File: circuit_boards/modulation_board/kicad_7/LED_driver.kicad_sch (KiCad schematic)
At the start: 11 parts

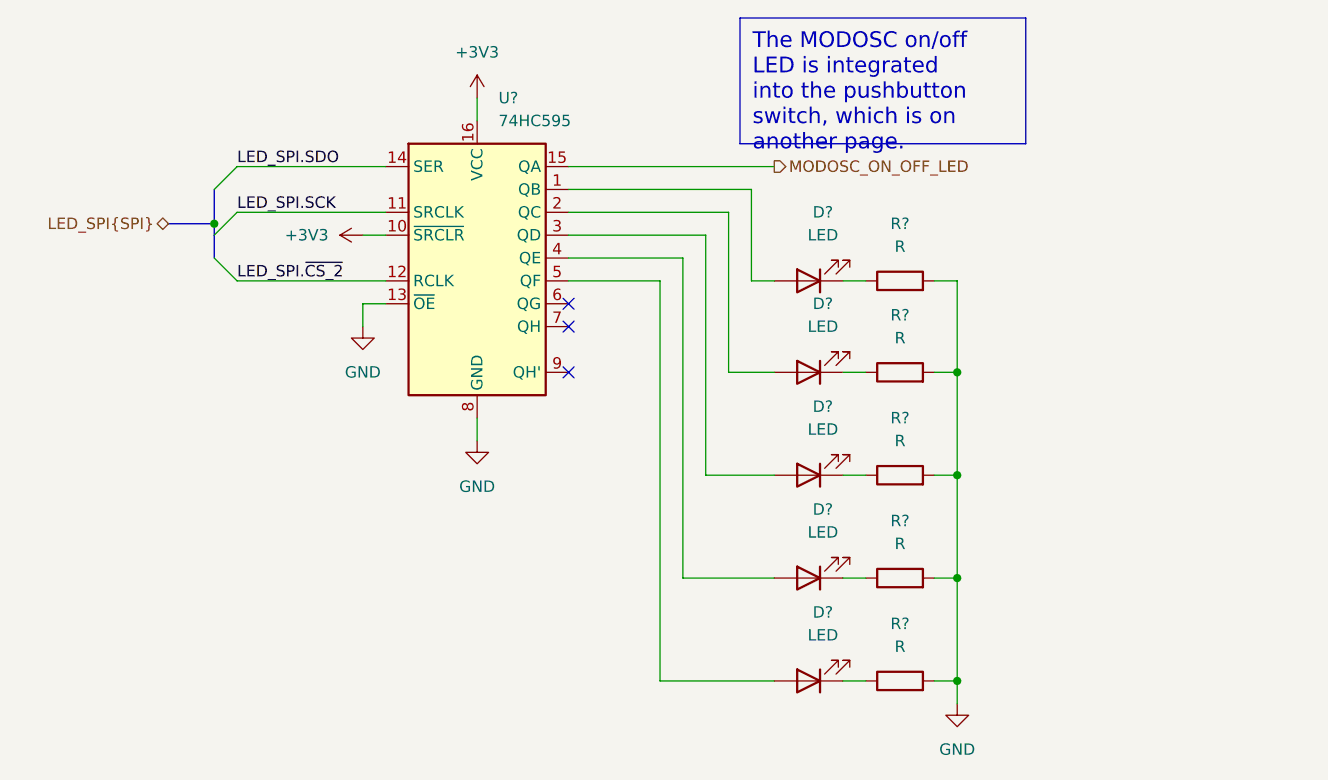
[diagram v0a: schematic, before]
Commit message: Progress on circuit boards
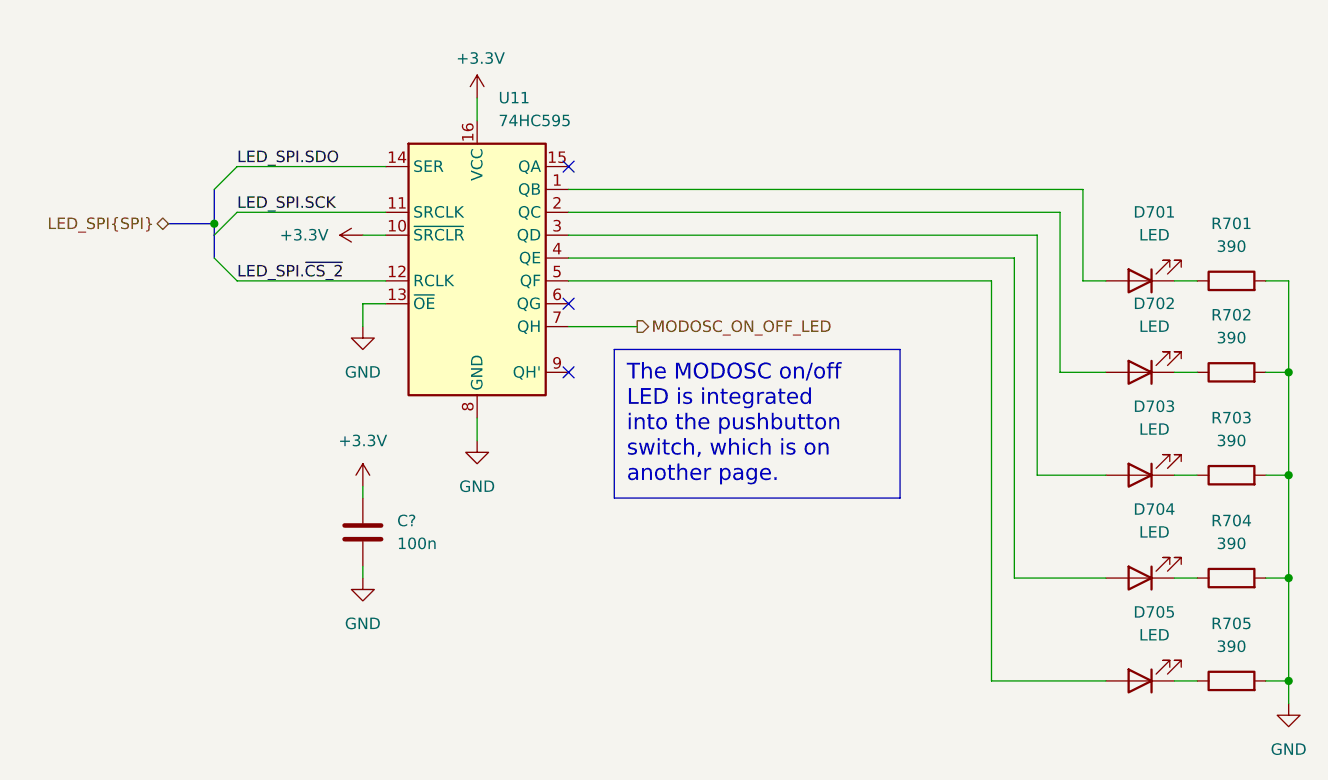
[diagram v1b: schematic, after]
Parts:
- added C?: 100n, Capacitor_SMD:C_0603_1608Metric, symbol Device:C
- D701, D702, D703, D704, D705: renamed from D?; footprint (none) -> LED_THT:LED_D3.0mm
- R701, R702, R703, R704, R705: renamed from R?; value R -> 390; footprint (none) -> Resistor_SMD:R_0603_1608Metric
- U11: renamed from U?; footprint (none) -> Package_SO:SOIC-16_3.9x9.9mm_P1.27mm
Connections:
- net GND: now also C?.2
- net MODOSC_ON_OFF_LED: now also U11.7 (QH); no longer U11.15 (QA)
- net +3V3 renamed +3.3V
- net +3.3V: now also C?.1
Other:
- moved on the sheet: D701, D702, D703, D704, D705, R701, R702, R703, R704, R705
